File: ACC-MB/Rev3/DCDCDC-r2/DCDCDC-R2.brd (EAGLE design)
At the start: 172 x 64 mm, 44 parts, among them P1330-102H 39uH

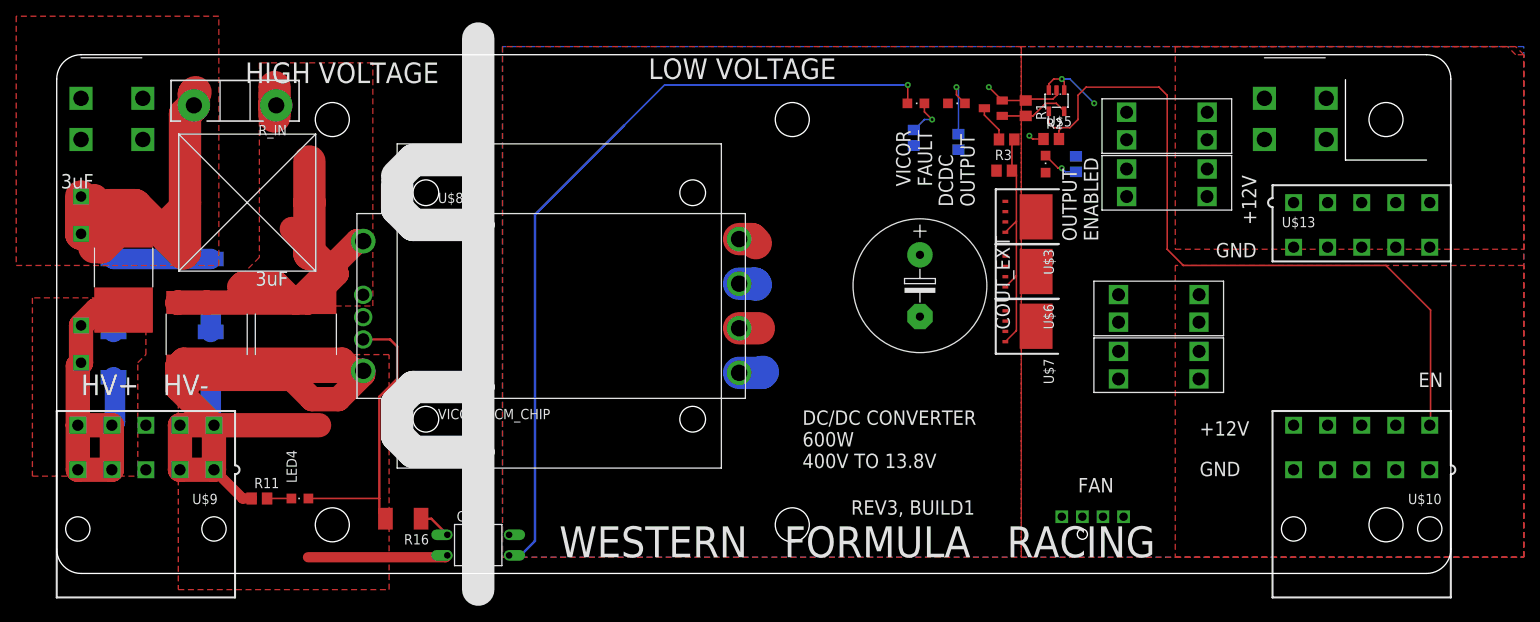
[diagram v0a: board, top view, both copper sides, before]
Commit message: update
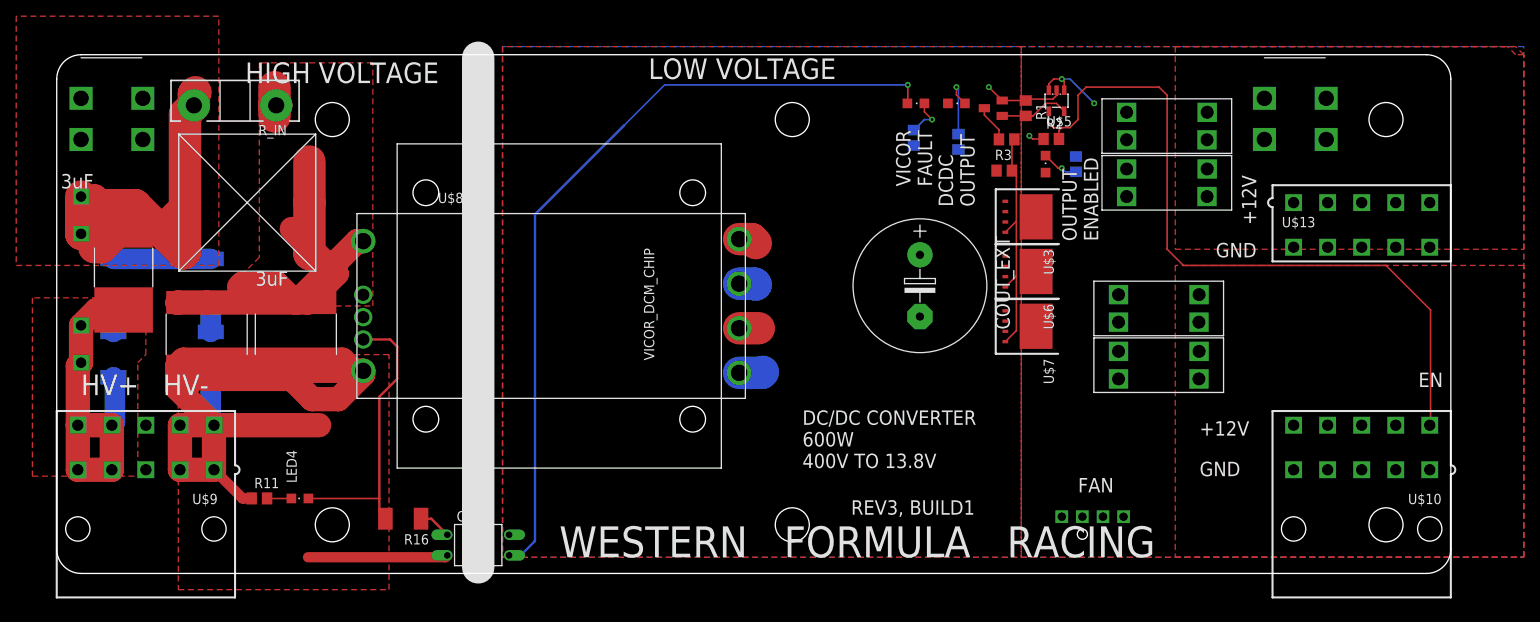
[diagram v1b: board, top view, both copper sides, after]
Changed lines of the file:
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@@
 <layer number="44" name="Drills" color="7" fill="1" visible="no" active="yes"/>
 <layer number="45" name="Holes" color="7" fill="1" visible="no" active="yes"/>
-<layer number="46" name="Milling" color="3" fill="1" visible="no" active="yes"/>
+<layer number="46" name="Milling" color="3" fill="1" visible="yes" active="yes"/>
 <layer number="47" name="Measures" color="7" fill="1" visible="no" active="yes"/>
 <layer number="48" name="Document" color="7" fill="1" visible="yes" active="yes"/>
@@
 <wire x1="3" y1="0" x2="169" y2="0" width="0" layer="20"/>
 <wire x1="172" y1="3" x2="172" y2="61" width="0" layer="20"/>
-<wire x1="52" y1="-2" x2="52" y2="15" width="4" layer="21"/>
 <dimension x1="50" y1="56" x2="54" y2="56" x3="52" y3="59" textsize="3.81" layer="21"/>
 <text x="23.25" y="60.5" size="2.54" layer="21">HIGH VOLTAGE</text>
@@
 <text x="62" y="2" size="3.81" layer="21">WESTERN   FORMULA   RACING</text>
 <text x="3" y="22" size="2.54" layer="21">HV+   HV-</text>
-<wire x1="52" y1="15" x2="52" y2="23" width="4" layer="21"/>
-<wire x1="52" y1="23" x2="52" y2="43" width="4" layer="21"/>
-<wire x1="52" y1="43" x2="52" y2="66" width="4" layer="21"/>
-<wire x1="52" y1="23" x2="44" y2="23" width="4" layer="21"/>
-<wire x1="44" y1="23" x2="42" y2="21" width="4" layer="21"/>
-<wire x1="42" y1="21" x2="42" y2="17" width="4" layer="21"/>
-<wire x1="42" y1="17" x2="44" y2="15" width="4" layer="21"/>
-<wire x1="44" y1="15" x2="52" y2="15" width="4" layer="21"/>
-<wire x1="51" y1="51" x2="44" y2="51" width="4" layer="21"/>
-<wire x1="44" y1="51" x2="42" y2="49" width="4" layer="21"/>
-<wire x1="42" y1="48" x2="42" y2="45" width="4" layer="21"/>
-<wire x1="42" y1="45" x2="44" y2="43" width="4" layer="21"/>
-<wire x1="44" y1="43" x2="52" y2="43" width="4" layer="21"/>
 <text x="98" y="7.25" size="1.778" layer="25">REV3, BUILD1</text>
 <text x="108" y="47.75" size="1.778" layer="25" rot="R90">VICOR
@@
 <text x="148" y="43" size="1.778" layer="25" rot="R90">+12V</text>
 <text x="126" y="10" size="1.778" layer="25">FAN</text>
+<wire x1="52" y1="63.625" x2="52" y2="0.75" width="4" layer="25"/>
+<wire x1="52.125" y1="0.875" x2="52.125" y2="63.75" width="4" layer="26"/>
 </plain>
 <attributes>
@@
 <element name="U$8" library="ACC-MB-R0" library_urn="urn:adsk.eagle:library:13208985" package="VICOR_CHIP_HEATSINK" package3d_urn="urn:adsk.eagle:package:13209498/4" value="VICOR_DCM_CHIP" x="61" y="33" smashed="yes">
 <attribute name="NAME" x="47.03" y="45.7" size="1.27" layer="21"/>
-<attribute name="VALUE" x="47.03" y="19.03" size="1.27" layer="21"/>
+<attribute name="VALUE" x="73.72" y="26.28" size="1.27" layer="21" rot="R90"/>
 </element>
 <element name="LED2" library="ACC-MB-R0" library_urn="urn:adsk.eagle:library:13208985" package="CHIPLED_0805" package3d_urn="urn:adsk.eagle:package:15821/2" value="" x="111" y="58" smashed="yes" rot="R270">
